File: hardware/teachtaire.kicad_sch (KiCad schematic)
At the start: 42 parts, among them J1 39-29-1048, J2 ESQ-110-X-X-D, J3 Conn_Coaxial, J4 5023860570, Q1 NMOS, Q2 IPD90P04P4L04ATMA1, U1 MAX-M10S, U2 STM32F072C8Tx, U3 TJA1051T/3/1J, U4 RF-LORA-868-SO

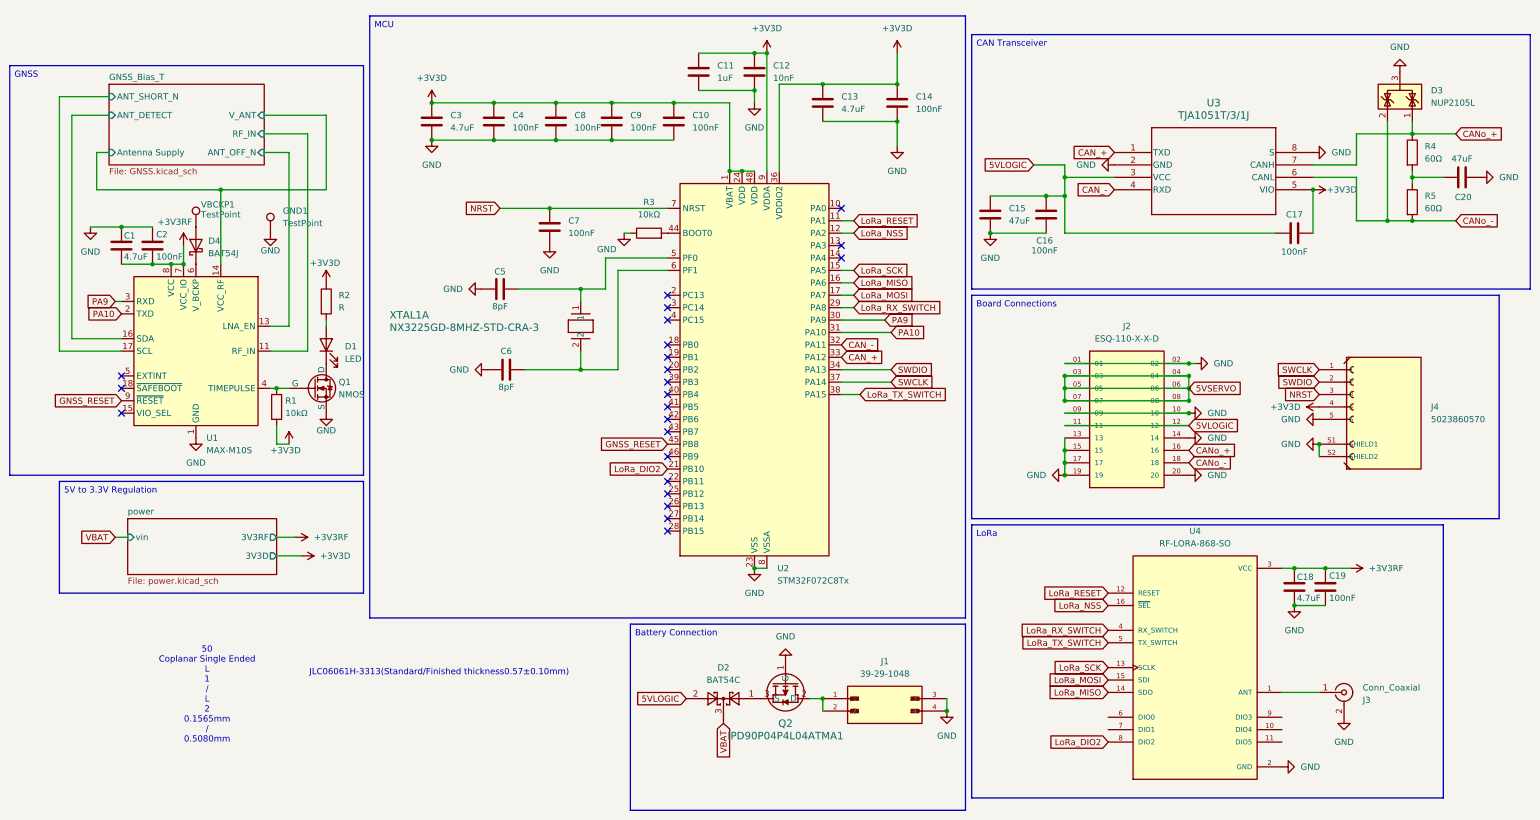
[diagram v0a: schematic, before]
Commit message: ddio pins
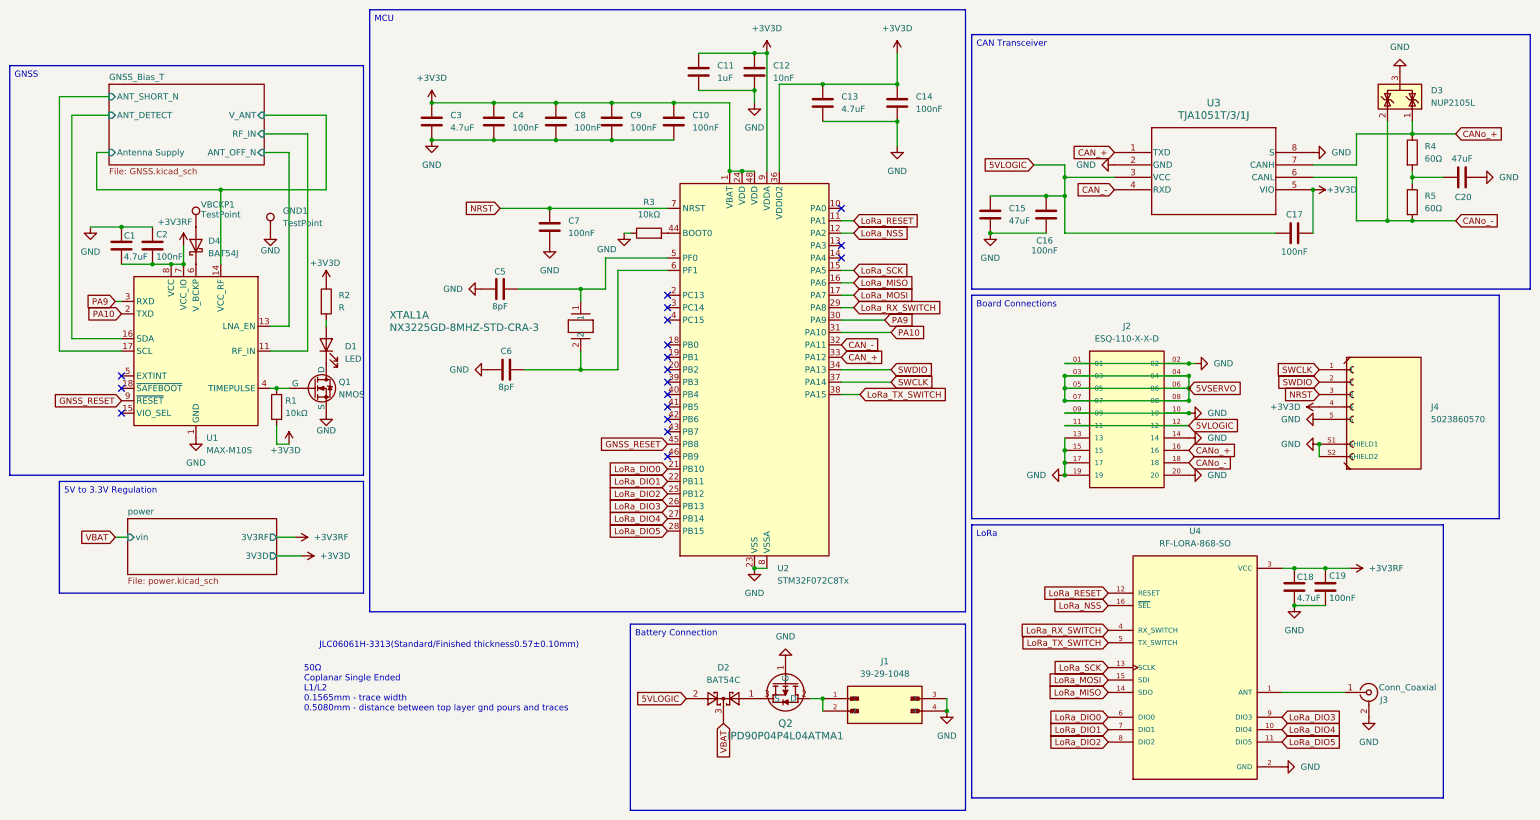
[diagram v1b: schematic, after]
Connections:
- net LoRa_DIO2: now also U2.25 (PB12); no longer U2.21 (PB10)
- net LoRa_DIO4: now reaches U4.10 (DIO4)
- net LoRa_DIO4: now also U2.27 (PB14)
- net LoRa_DIO5: now reaches U4.11 (DIO5)
- net LoRa_DIO5: now also U2.28 (PB15)
- net LoRa_DIO0: now reaches U4.6 (DIO0)
- net LoRa_DIO0: now also U2.21 (PB10)
- net LoRa_DIO1: now reaches U4.7 (DIO1)
- net LoRa_DIO1: now also U2.22 (PB11)
- net LoRa_DIO3: now reaches U4.9 (DIO3)
- net LoRa_DIO3: now also U2.26 (PB13)
- no-connect marks 23 -> 18
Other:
- note added: "50Ω Coplanar Single Ended L1/L2 0.1565mm - trace width 0.5080mm - distance between top layer gnd pours and traces"
- note removed: "50 Coplanar Single Ended L 1 / L 2 0.1565mm / 0.5080mm"
- moved on the sheet: J3
